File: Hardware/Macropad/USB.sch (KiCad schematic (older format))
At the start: 18 parts, among them J1 USB_C_Receptacle_USB2.0, U1 TCR2EF33, U2 SRV05-4

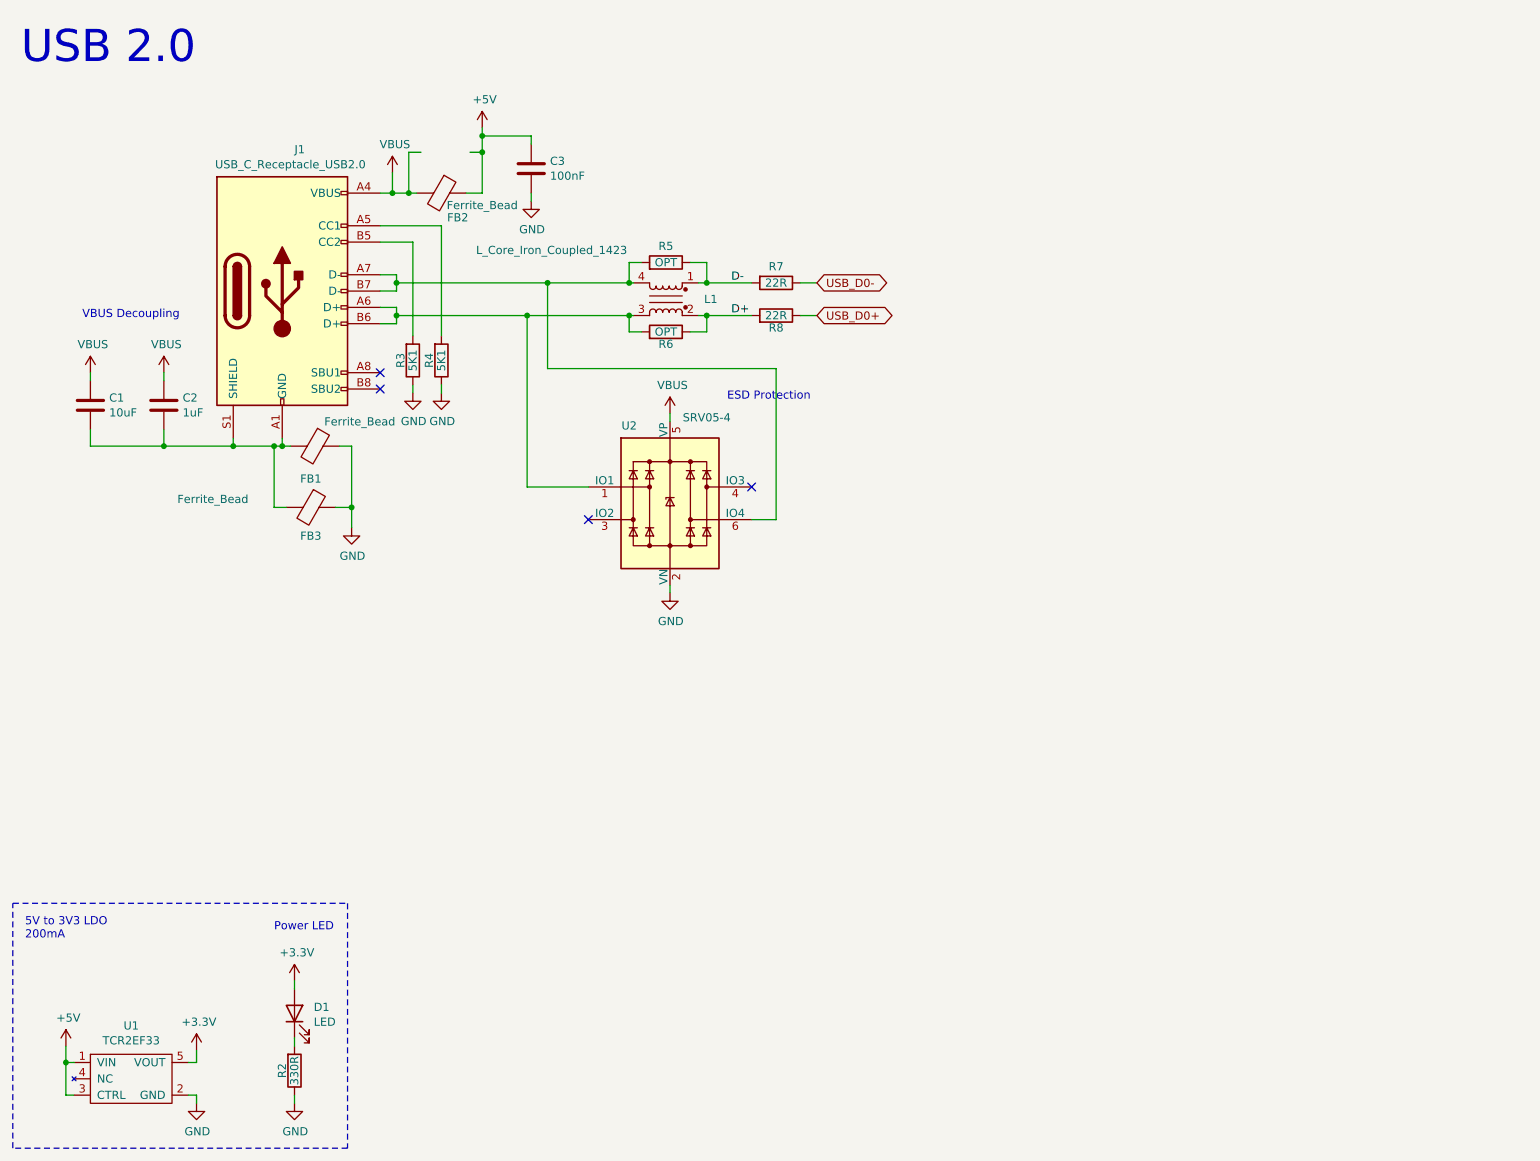
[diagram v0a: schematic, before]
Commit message: Layout done, cleaned up schematic and generated gerbers
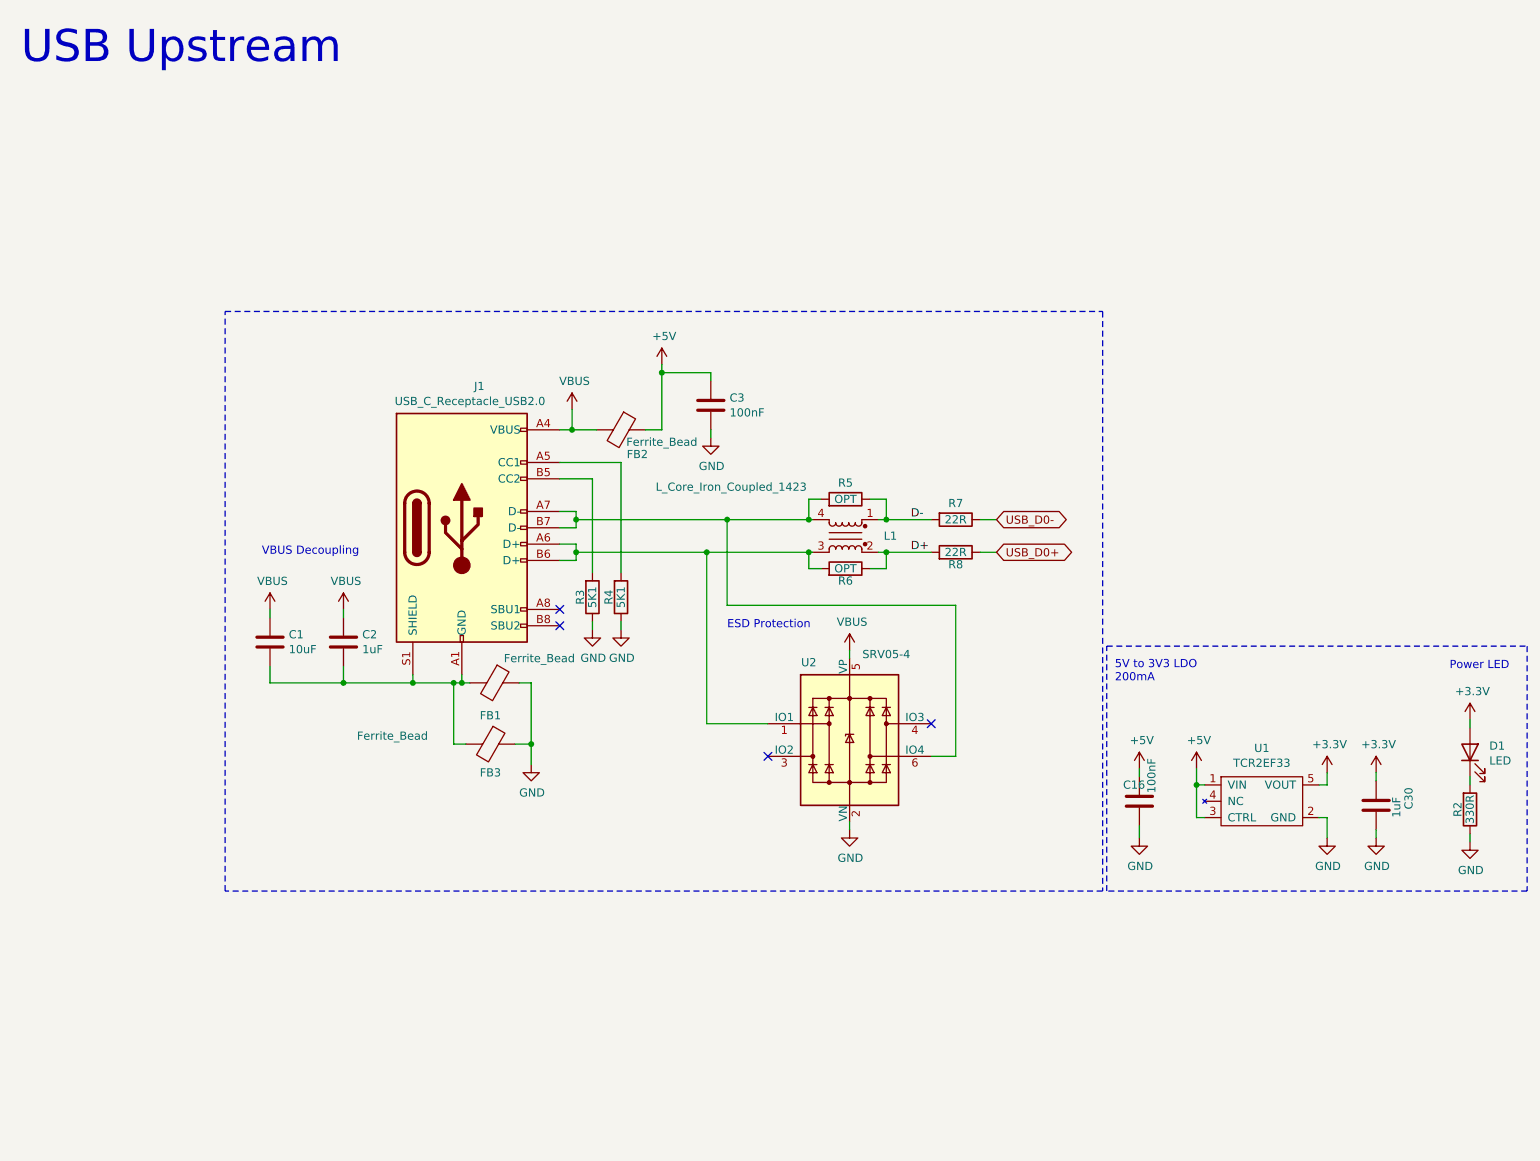
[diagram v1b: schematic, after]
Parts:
- added C16: 100nF, Capacitor_smd:C_0603_1608Metric, symbol Device:C
- added C30: 1uF, Capacitor_smd:C_0603_1608Metric, symbol Device:C
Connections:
- net +3V3: now also C30.1
- net +5V: now also C16.1
- net GND: now also C16.2, C30.2
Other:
- note added: "USB Upstream"
- note removed: "USB 2.0"
- moved on the sheet: C1, C2, C3, D1, FB1, FB2, FB3, J1, L1, R2, R3, R4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
